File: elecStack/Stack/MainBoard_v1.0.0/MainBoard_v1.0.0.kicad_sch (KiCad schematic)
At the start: 26 parts, among them J1 Conn_01x04_Socket, J2 Conn_01x06_Pin, J3 Conn_01x06_Pin, Q1 NMOS, Q2 NMOS, Q3 NMOS, Q4 NMOS, Q5 NMOS, Q6 NMOS, Q7 NMOS, Q8 PMOS, U1 RASPBERRY_PI_PICO, U2 L293D, U3 TXS0108EPW, U4 L293D

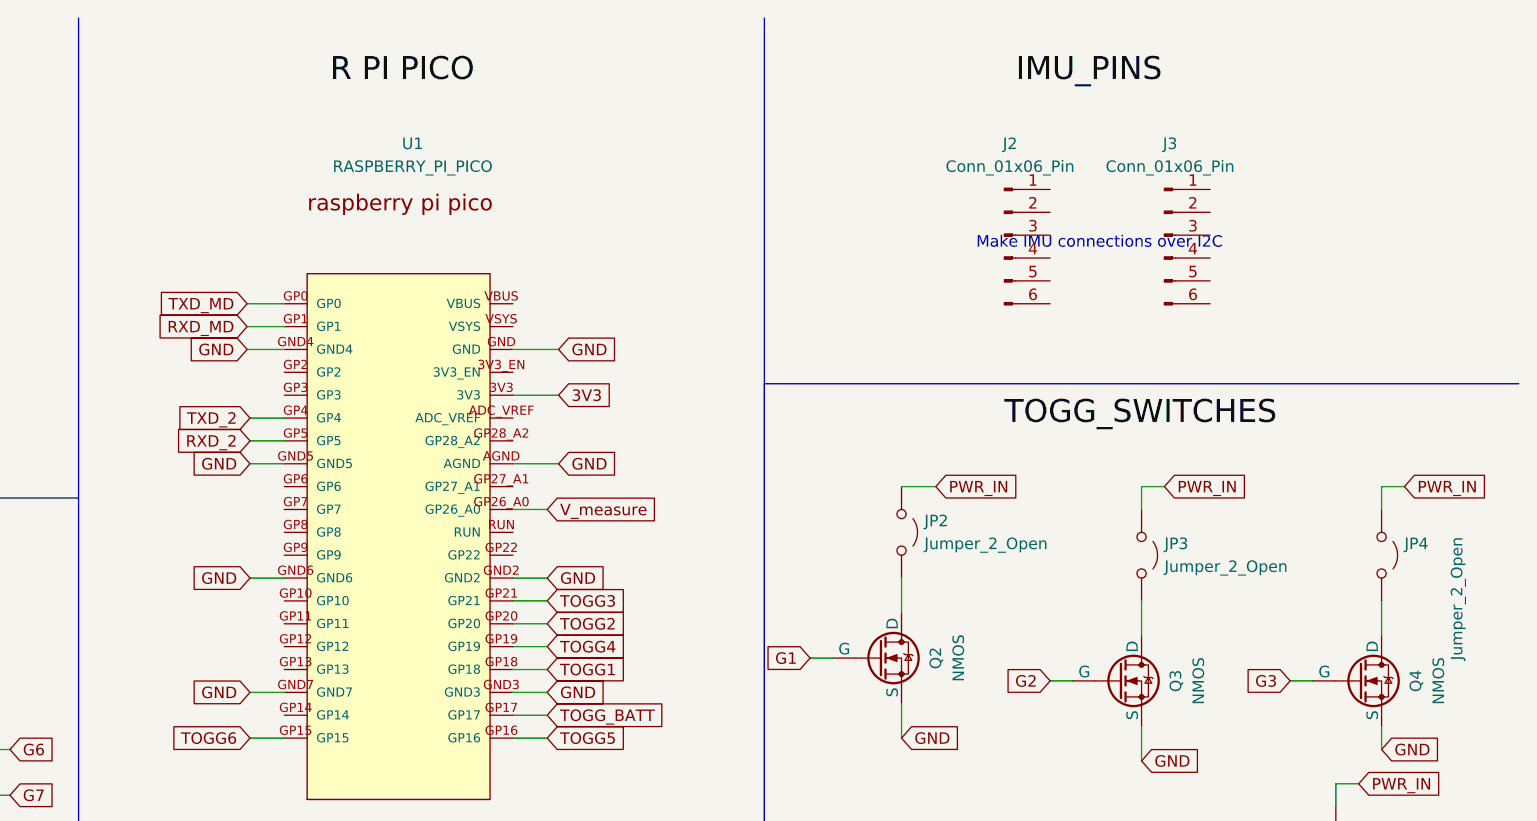
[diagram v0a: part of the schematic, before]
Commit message: IMU_connected
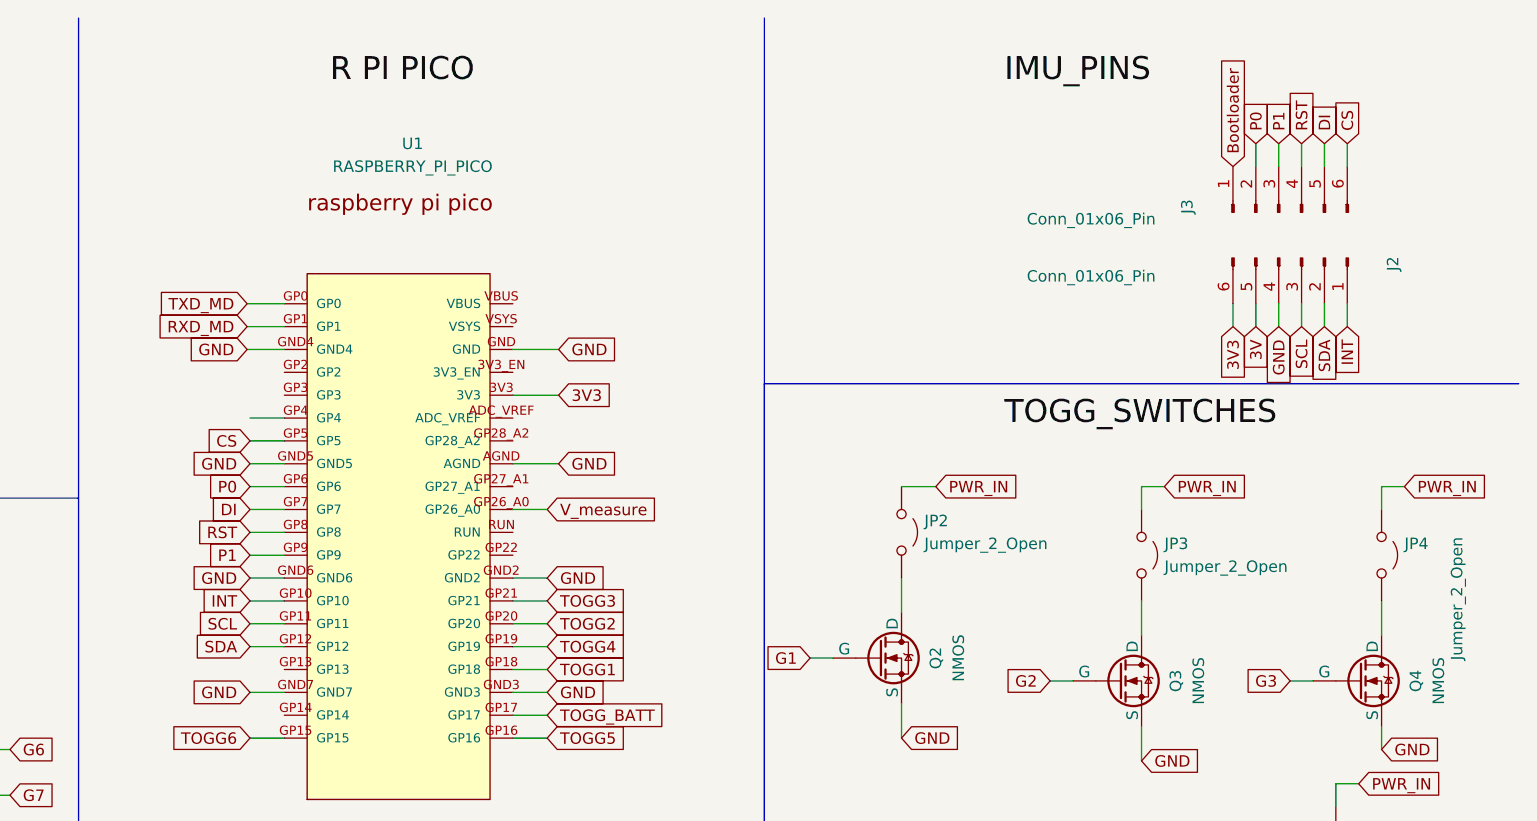
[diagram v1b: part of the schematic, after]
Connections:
- net RXD_2 is gone; now on net CS: U1.GP5
- net 3V3: now also J2.6 (Pin_6)
- net GND: now also J2.4 (Pin_4)
- net INT: now reaches U1.GP10
- net INT: now also J2.1 (Pin_1)
- net SCL: now reaches U1.GP11
- net SCL: now also J2.3 (Pin_3)
- net SDA: now reaches U1.GP12
- net SDA: now also J2.2 (Pin_2)
- net P0: now reaches U1.GP6
- net P0: now also J3.2 (Pin_2)
- net DI: now reaches U1.GP7
- net DI: now also J3.5 (Pin_5)
- net RST: now reaches U1.GP8
- net RST: now also J3.4 (Pin_4)
- net P1: now reaches U1.GP9
- net P1: now also J3.3 (Pin_3)
- net Bootloader: now reaches J3.1 (Pin_1)
- net CS: now reaches J3.6 (Pin_6)
- net 3V: now reaches J2.5 (Pin_5)
- net TXD_2: no longer names the net of U1.GP4
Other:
- note removed: "Make IMU connections over I2C"
- moved on the sheet: J2, J3
